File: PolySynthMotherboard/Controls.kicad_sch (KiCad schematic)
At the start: 92 parts, among them SW601 ENV1_B, SW602 ENV2_B, SW603 LFO1_B, SW604 LFO2_B, SW605 LFO3_B, SW606 MIX1_B, SW607 MIX2_B, SW608 MENU_B, SW609 FF_B, SW610 HP_B, SW611 HP_B, U204 ILI9341, U501 MCP23S17_SS

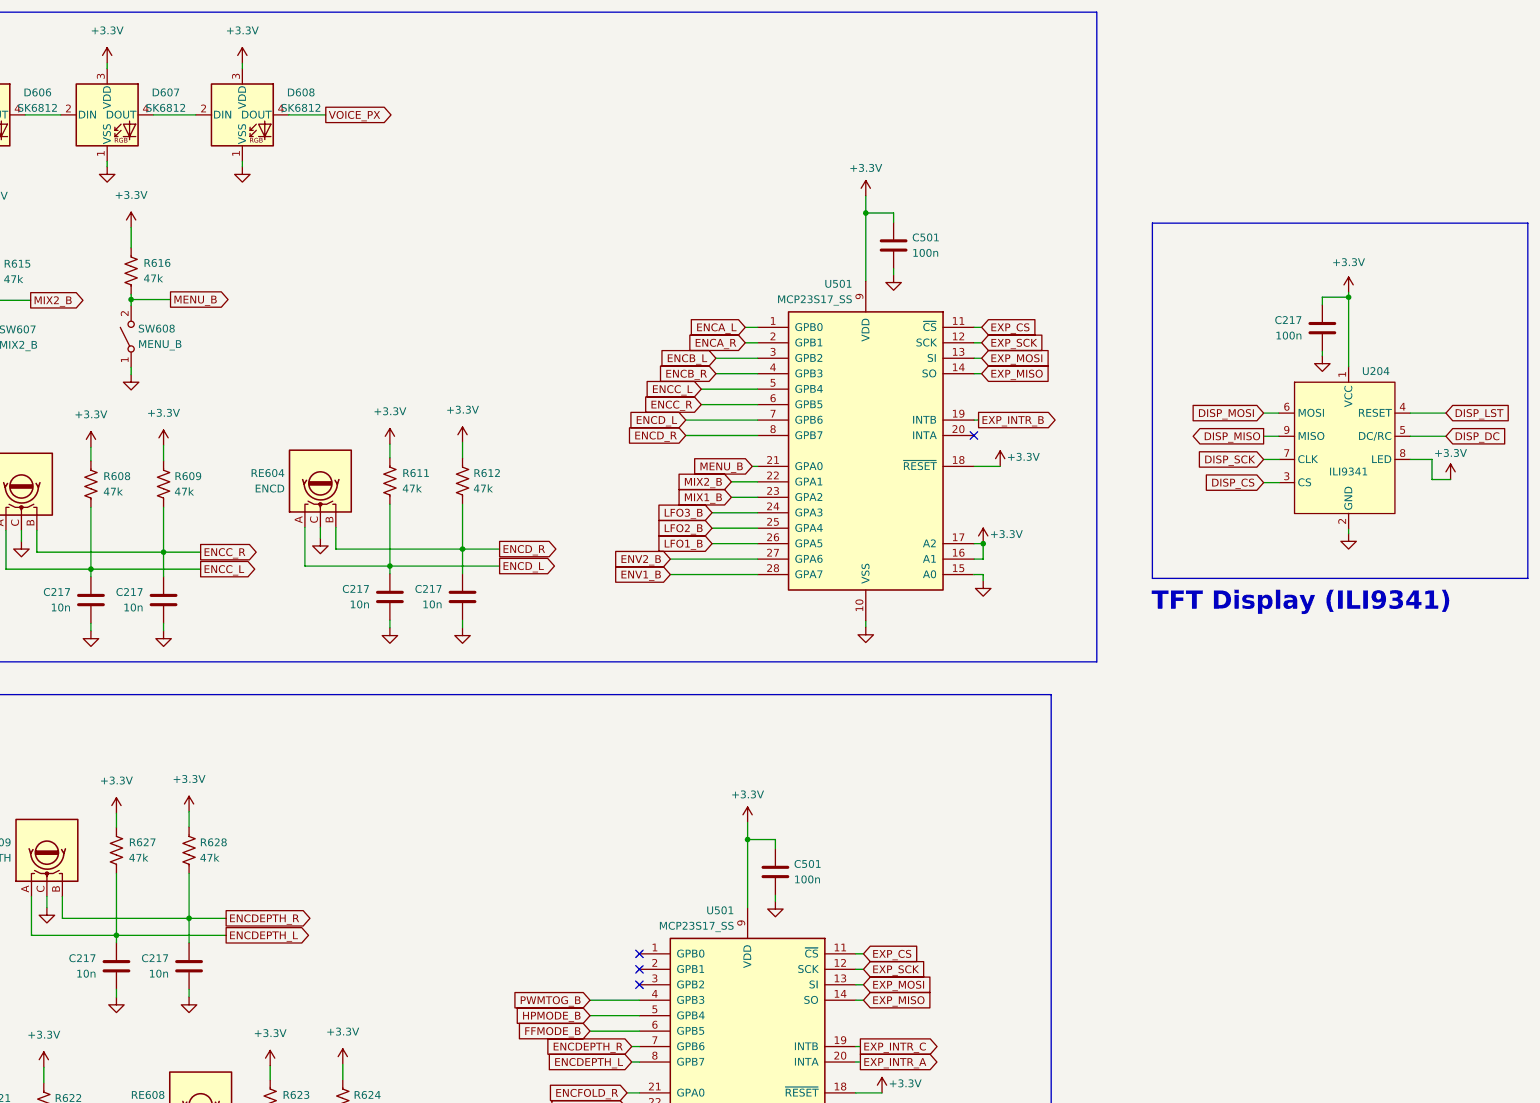
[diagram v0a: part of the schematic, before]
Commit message: fixed git maybe
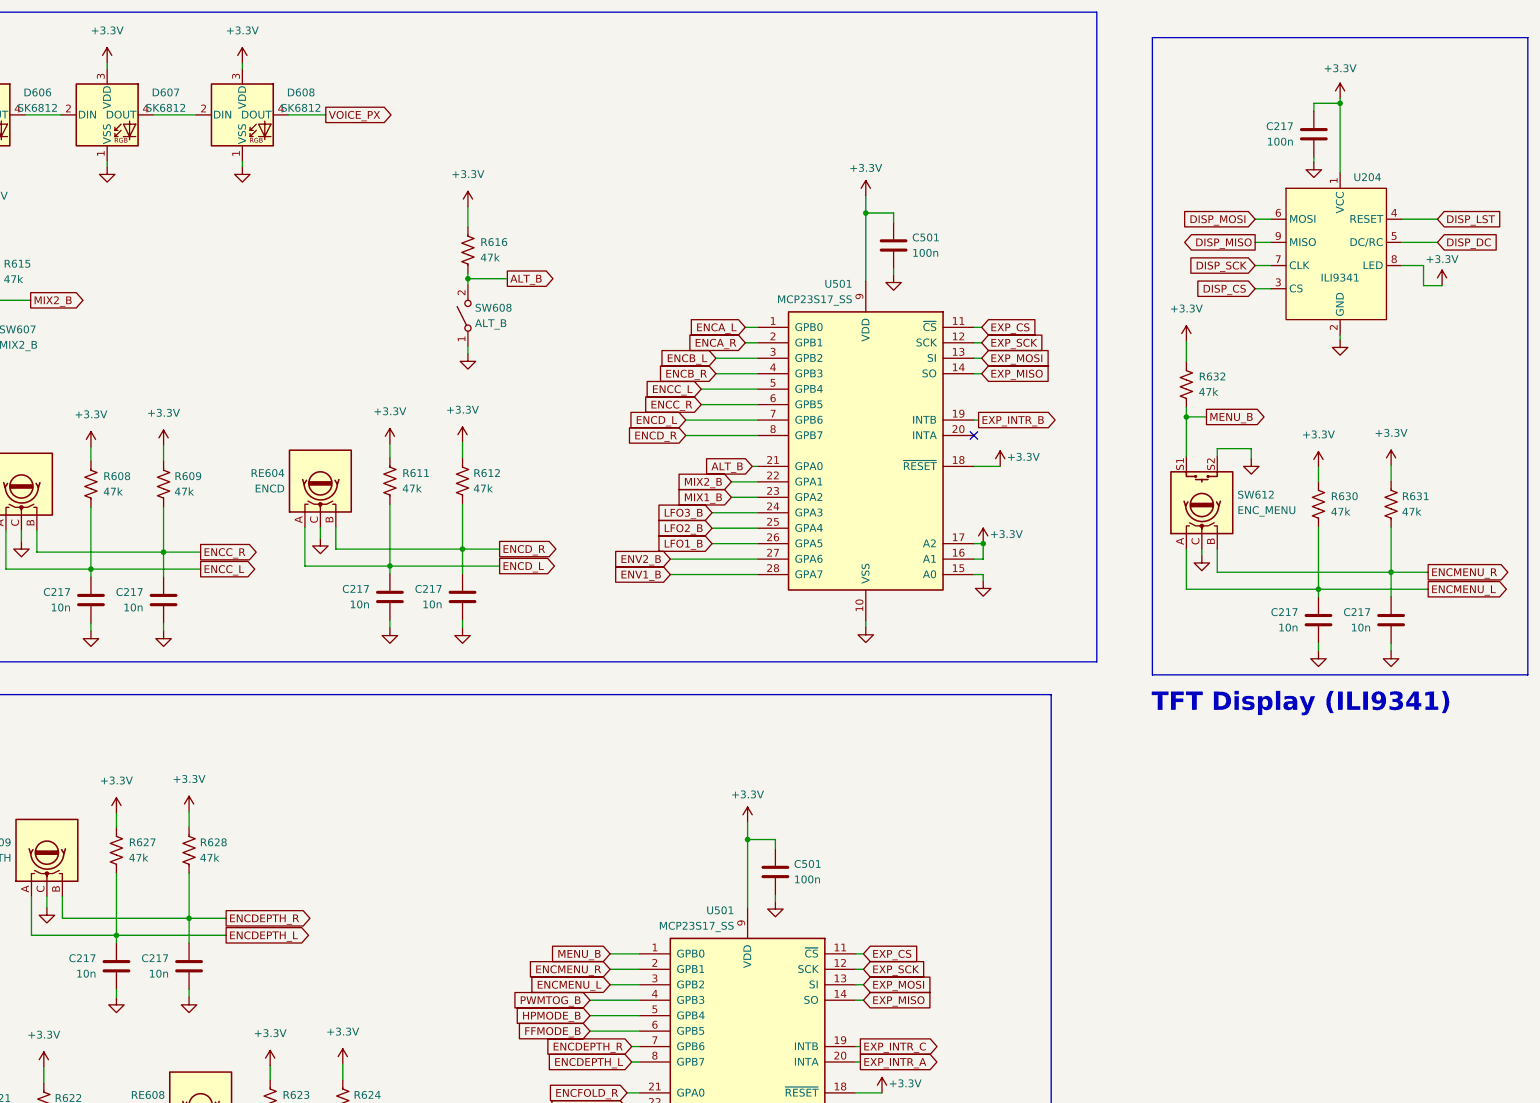
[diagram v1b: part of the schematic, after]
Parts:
- added C217 (x2): 10n, Capacitor_SMD:C_0805_2012Metric, symbol Device:C
- added R630, R631, R632: 47k, PCM_Resistor_SMD_AKL:R_0805_2012Metric, symbol Device:R_US
- added SW612: ENC_MENU, Alps_Rotary_Encoder:RotaryEncoder_Alps_EC11E-Switch_Vertical_H20mm_5Pin, symbol Device:RotaryEncoder_Switch
- SW608: value MENU_B -> ALT_B
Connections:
- net +3.3V: now also R630.1, R631.1, R632.1
- net GND: now also C217.2, C217.2, SW612.C, SW612.S2
- net MENU_B: now also U501.1 (GPB0), R632.2, SW612.S1; no longer R616.2, SW608.2 (B), U501.21 (GPA0)
- net ENCMENU_R: now reaches U501.2 (GPB1)
- net ENCMENU_R: now also C217.1, R631.2, SW612.B
- net ENCMENU_L: now reaches U501.3 (GPB2)
- net ENCMENU_L: now also C217.1, R630.2, SW612.A
- new net ALT_B: R616.2, SW608.2 (B), U501.21 (GPA0)
- no-connect marks 5 -> 2
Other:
- moved on the sheet: C217, R616, SW608, U204
